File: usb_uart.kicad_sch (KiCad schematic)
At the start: 10 parts

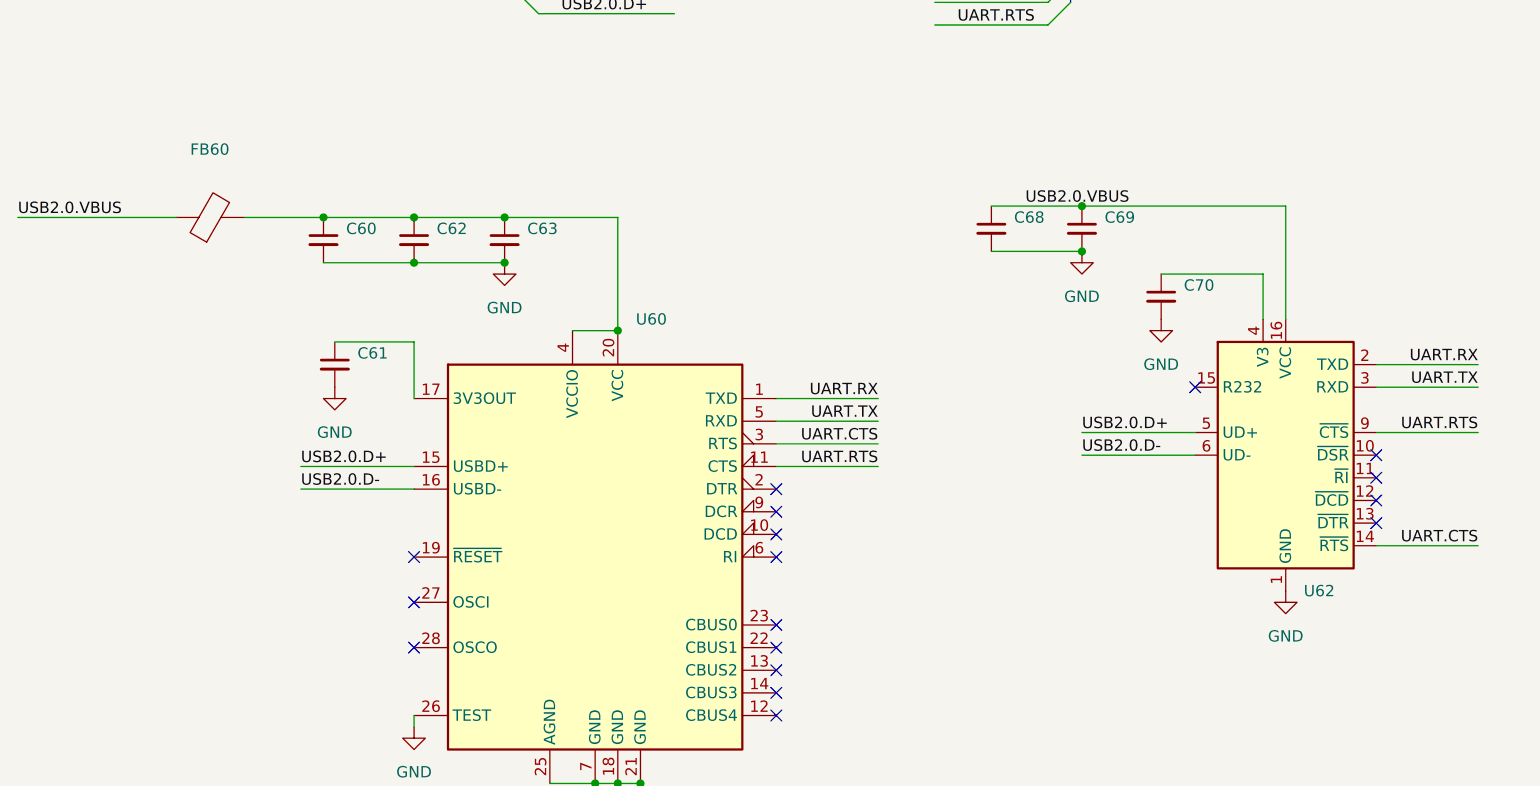
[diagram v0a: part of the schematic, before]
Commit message: Add heatsink, among other things
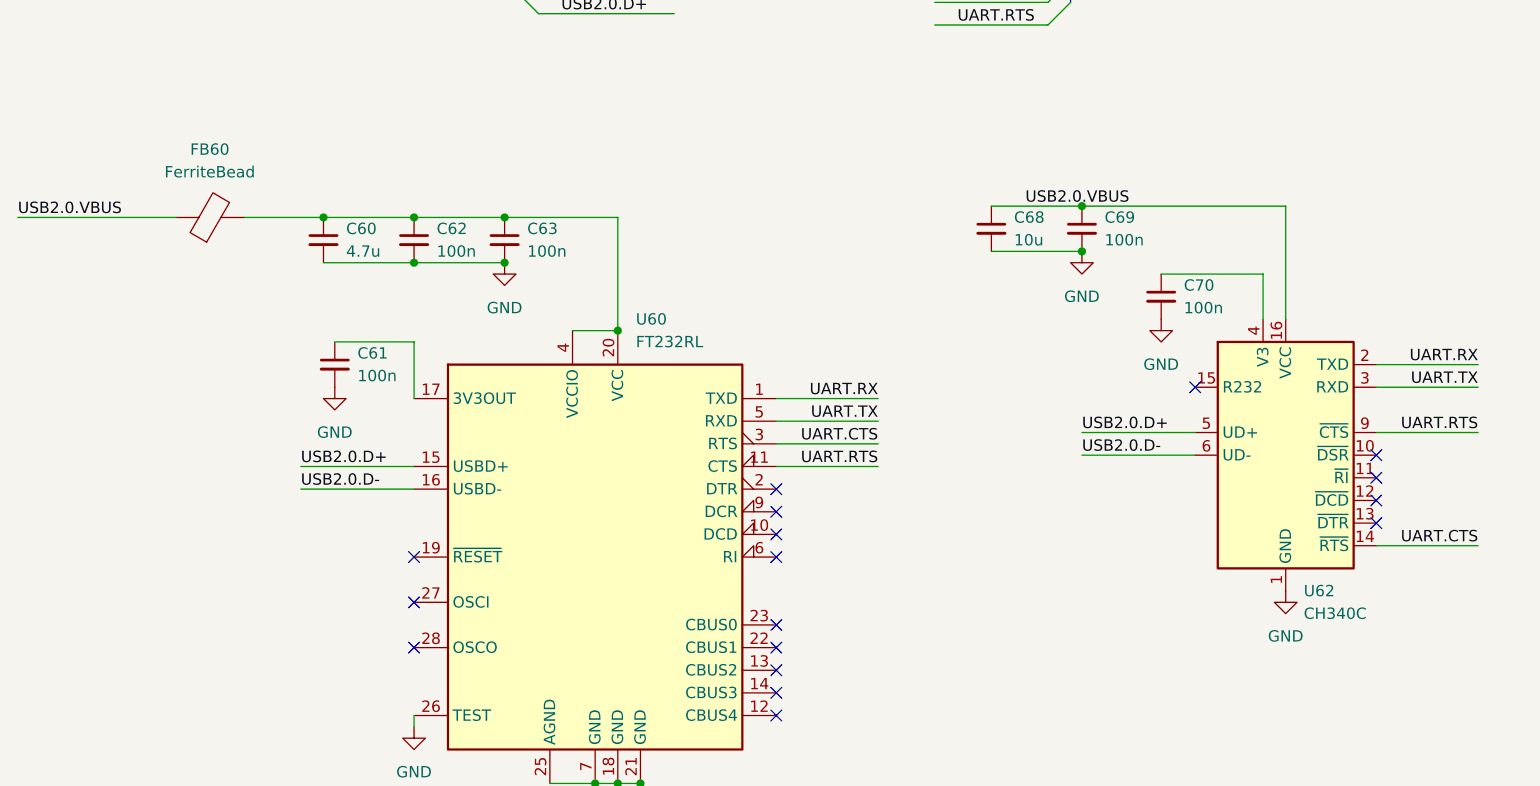
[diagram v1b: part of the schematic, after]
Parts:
- C60: value (none) -> 4.7u; footprint (none) -> Capacitor_SMD:C_0805_2012Metric
- C61, C62, C63, C69, C70: value (none) -> 100n; footprint (none) -> Capacitor_SMD:C_0402_1005Metric
- C68: value (none) -> 10u; footprint (none) -> Capacitor_SMD:C_0805_2012Metric
- FB60: value (none) -> FerriteBead; footprint (none) -> Inductor_SMD:L_0805_2012Metric
- U60: value (none) -> FT232RL; footprint (none) -> Package_SO:SSOP-28_5.3x10.2mm_P0.65mm
- U62: value (none) -> CH340C; footprint (none) -> Package_SO:SOIC-16_3.9x9.9mm_P1.27mm
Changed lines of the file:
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@@
       (effects (font (size 1.27 1.27)) (justify left))
     )
-    (property "Value" "" (id 1) (at 76.2 88.9062 0)
-      (effects (font (size 1.27 1.27)) (justify left))
-    )
-    (property "Footprint" "" (id 2) (at 73.66 87.63 0)
+    (property "Value" "100n" (id 1) (at 76.2 88.9062 0)
+      (effects (font (size 1.27 1.27)) (justify left))
+    )
+    (property "Footprint" "Capacitor_SMD:C_0402_1005Metric" (id 2) (at 73.66 87.63 0)
       (effects (font (size 1.27 1.27)) hide)
     )
@@
       (effects (font (size 1.27 1.27)) (justify left))
     )
-    (property "Value" "" (id 1) (at 107.4294 85.09 0)
-      (effects (font (size 1.27 1.27)) (justify left))
-    )
-    (property "Footprint" "" (id 2) (at 130.81 132.08 0)
+    (property "Value" "FT232RL" (id 1) (at 107.4294 85.09 0)
+      (effects (font (size 1.27 1.27)) (justify left))
+    )
+    (property "Footprint" "Package_SO:SSOP-28_5.3x10.2mm_P0.65mm" (id 2) (at 130.81 132.08 0)
       (effects (font (size 1.27 1.27)) hide)
     )
@@
       (effects (font (size 1.27 1.27)) (justify left))
     )
-    (property "Value" "" (id 1) (at 182.3594 115.57 0)
-      (effects (font (size 1.27 1.27)) (justify left))
-    )
-    (property "Footprint" "" (id 2) (at 181.61 111.76 0)
+    (property "Value" "CH340C" (id 1) (at 182.3594 115.57 0)
+      (effects (font (size 1.27 1.27)) (justify left))
+    )
+    (property "Footprint" "Package_SO:SOIC-16_3.9x9.9mm_P1.27mm" (id 2) (at 181.61 111.76 0)
       (effects (font (size 1.27 1.27)) (justify left) hide)
     )
@@
       (effects (font (size 1.27 1.27)) (justify left))
     )
-    (property "Value" "" (id 1) (at 85.09 74.9362 0)
-      (effects (font (size 1.27 1.27)) (justify left))
-    )
-    (property "Footprint" "" (id 2) (at 82.55 73.66 0)
+    (property "Value" "100n" (id 1) (at 85.09 74.9362 0)
+      (effects (font (size 1.27 1.27)) (justify left))
+    )
+    (property "Footprint" "Capacitor_SMD:C_0402_1005Metric" (id 2) (at 82.55 73.66 0)
       (effects (font (size 1.27 1.27)) hide)
     )
@@
       (effects (font (size 1.27 1.27)) (justify left))
     )
-    (property "Value" "" (id 1) (at 168.91 81.2862 0)
-      (effects (font (size 1.27 1.27)) (justify left))
-    )
-    (property "Footprint" "" (id 2) (at 166.37 80.01 0)
+    (property "Value" "100n" (id 1) (at 168.91 81.2862 0)
+      (effects (font (size 1.27 1.27)) (justify left))
+    )
+    (property "Footprint" "Capacitor_SMD:C_0402_1005Metric" (id 2) (at 166.37 80.01 0)
       (effects (font (size 1.27 1.27)) hide)
     )
@@
       (effects (font (size 1.27 1.27)) (justify left))
     )
-    (property "Value" "" (id 1) (at 149.86 73.6662 0)
-      (effects (font (size 1.27 1.27)) (justify left))
-    )
-    (property "Footprint" "" (id 2) (at 147.32 72.39 0)
+    (property "Value" "10u" (id 1) (at 149.86 73.6662 0)
+      (effects (font (size 1.27 1.27)) (justify left))
+    )
+    (property "Footprint" "Capacitor_SMD:C_0805_2012Metric" (id 2) (at 147.32 72.39 0)
       (effects (font (size 1.27 1.27)) hide)
     )
@@
       (effects (font (size 1.27 1.27)) (justify left))
     )
-    (property "Value" "" (id 1) (at 160.02 73.6662 0)
-      (effects (font (size 1.27 1.27)) (justify left))
-    )
-    (property "Footprint" "" (id 2) (at 157.48 72.39 0)
+    (property "Value" "100n" (id 1) (at 160.02 73.6662 0)
+      (effects (font (size 1.27 1.27)) (justify left))
+    )
+    (property "Footprint" "Capacitor_SMD:C_0402_1005Metric" (id 2) (at 157.48 72.39 0)
       (effects (font (size 1.27 1.27)) hide)
     )
@@
       (effects (font (size 1.27 1.27)) (justify left))
     )
-    (property "Value" "" (id 1) (at 95.25 74.9362 0)
-      (effects (font (size 1.27 1.27)) (justify left))
-    )
-    (property "Footprint" "" (id 2) (at 92.71 73.66 0)
+    (property "Value" "100n" (id 1) (at 95.25 74.9362 0)
+      (effects (font (size 1.27 1.27)) (justify left))
+    )
+    (property "Footprint" "Capacitor_SMD:C_0402_1005Metric" (id 2) (at 92.71 73.66 0)
       (effects (font (size 1.27 1.27)) hide)
     )
@@
       (effects (font (size 1.27 1.27)) (justify left))
     )
-    (property "Value" "" (id 1) (at 74.93 74.9362 0)
-      (effects (font (size 1.27 1.27)) (justify left))
-    )
-    (property "Footprint" "" (id 2) (at 72.39 73.66 0)
+    (property "Value" "4.7u" (id 1) (at 74.93 74.9362 0)
+      (effects (font (size 1.27 1.27)) (justify left))
+    )
+    (property "Footprint" "Capacitor_SMD:C_0805_2012Metric" (id 2) (at 72.39 73.66 0)
       (effects (font (size 1.27 1.27)) hide)
     )
@@
     (in_bom yes) (on_board yes) (fields_autoplaced)
     (property "Reference" "FB60" (id 0) (at 59.6392 63.5 90))
-    (property "Value" "" (id 1) (at 59.6392 66.04 90))
-    (property "Footprint" "" (id 2) (at 59.69 72.898 90)
-      (effects (font (size 1.27 1.27)) hide)
-    )
+    (property "Value" "FerriteBead" (id 1) (at 59.6392 66.04 90))
+    (property "Footprint" "Inductor_SMD:L_0805_2012Metric" (id 2) (at 59.69 72.898 90)
+      (effects (font (size 1.27 1.27)) hide)
+    )

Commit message: WIP PCB Routing
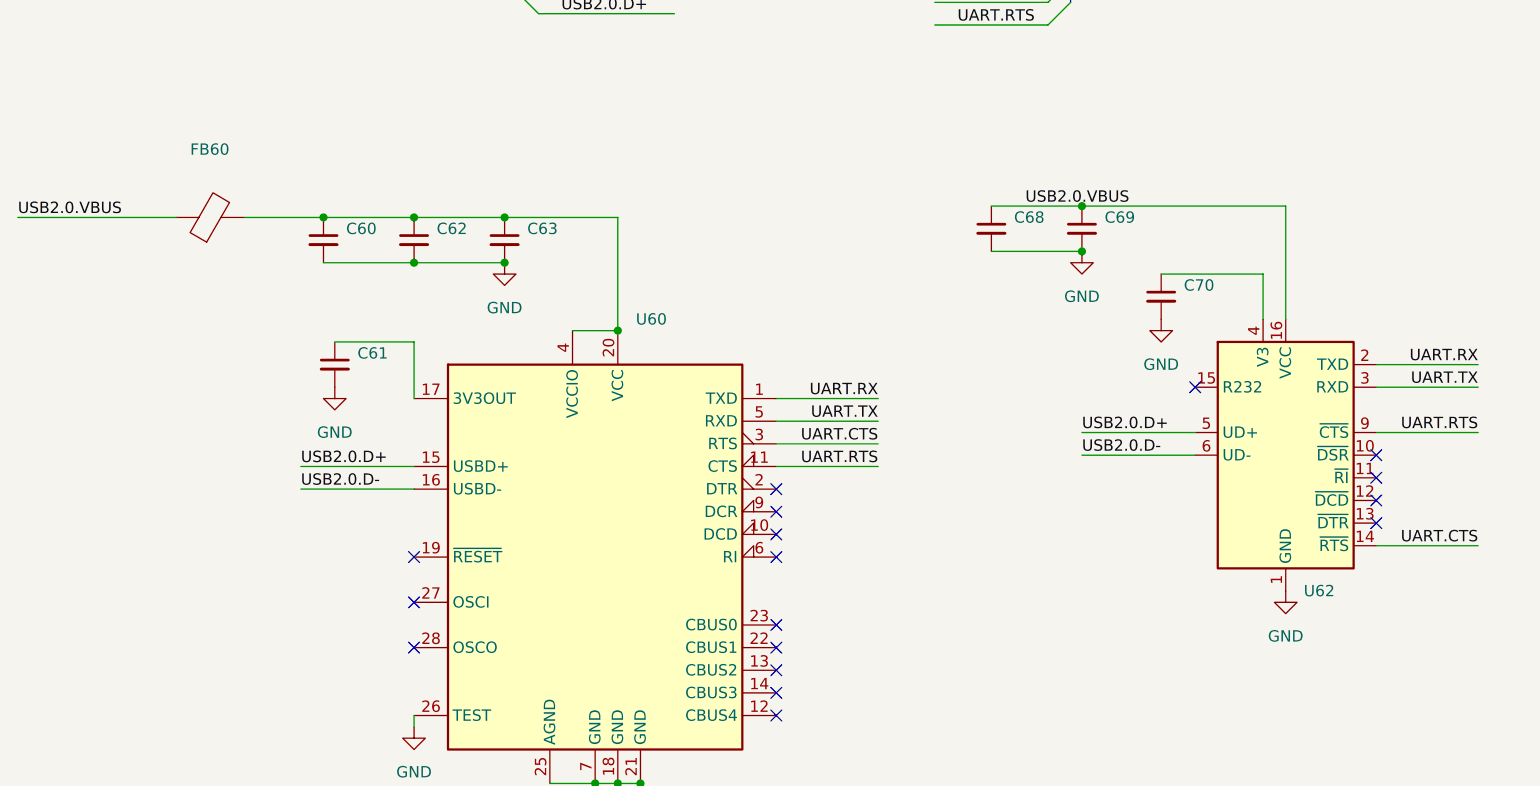
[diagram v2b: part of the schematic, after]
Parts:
- C60: value 4.7u -> (none); footprint Capacitor_SMD:C_0805_2012Metric -> (none)
- C61, C62, C63, C69, C70: value 100n -> (none); footprint Capacitor_SMD:C_0402_1005Metric -> (none)
- C68: value 10u -> (none); footprint Capacitor_SMD:C_0805_2012Metric -> (none)
- FB60: value FerriteBead -> (none); footprint Inductor_SMD:L_0805_2012Metric -> (none)
- U60: value FT232RL -> (none); footprint Package_SO:SSOP-28_5.3x10.2mm_P0.65mm -> (none)
- U62: value CH340C -> (none); footprint Package_SO:SOIC-16_3.9x9.9mm_P1.27mm -> (none)
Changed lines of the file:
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@@
       (effects (font (size 1.27 1.27)) (justify left))
     )
-    (property "Value" "100n" (id 1) (at 76.2 88.9062 0)
-      (effects (font (size 1.27 1.27)) (justify left))
-    )
-    (property "Footprint" "Capacitor_SMD:C_0402_1005Metric" (id 2) (at 73.66 87.63 0)
+    (property "Value" "" (id 1) (at 76.2 88.9062 0)
+      (effects (font (size 1.27 1.27)) (justify left))
+    )
+    (property "Footprint" "" (id 2) (at 73.66 87.63 0)
       (effects (font (size 1.27 1.27)) hide)
     )
@@
       (effects (font (size 1.27 1.27)) (justify left))
     )
-    (property "Value" "FT232RL" (id 1) (at 107.4294 85.09 0)
-      (effects (font (size 1.27 1.27)) (justify left))
-    )
-    (property "Footprint" "Package_SO:SSOP-28_5.3x10.2mm_P0.65mm" (id 2) (at 130.81 132.08 0)
+    (property "Value" "" (id 1) (at 107.4294 85.09 0)
+      (effects (font (size 1.27 1.27)) (justify left))
+    )
+    (property "Footprint" "" (id 2) (at 130.81 132.08 0)
       (effects (font (size 1.27 1.27)) hide)
     )
@@
       (effects (font (size 1.27 1.27)) (justify left))
     )
-    (property "Value" "CH340C" (id 1) (at 182.3594 115.57 0)
-      (effects (font (size 1.27 1.27)) (justify left))
-    )
-    (property "Footprint" "Package_SO:SOIC-16_3.9x9.9mm_P1.27mm" (id 2) (at 181.61 111.76 0)
+    (property "Value" "" (id 1) (at 182.3594 115.57 0)
+      (effects (font (size 1.27 1.27)) (justify left))
+    )
+    (property "Footprint" "" (id 2) (at 181.61 111.76 0)
       (effects (font (size 1.27 1.27)) (justify left) hide)
     )
@@
       (effects (font (size 1.27 1.27)) (justify left))
     )
-    (property "Value" "100n" (id 1) (at 85.09 74.9362 0)
-      (effects (font (size 1.27 1.27)) (justify left))
-    )
-    (property "Footprint" "Capacitor_SMD:C_0402_1005Metric" (id 2) (at 82.55 73.66 0)
+    (property "Value" "" (id 1) (at 85.09 74.9362 0)
+      (effects (font (size 1.27 1.27)) (justify left))
+    )
+    (property "Footprint" "" (id 2) (at 82.55 73.66 0)
       (effects (font (size 1.27 1.27)) hide)
     )
@@
       (effects (font (size 1.27 1.27)) (justify left))
     )
-    (property "Value" "100n" (id 1) (at 168.91 81.2862 0)
-      (effects (font (size 1.27 1.27)) (justify left))
-    )
-    (property "Footprint" "Capacitor_SMD:C_0402_1005Metric" (id 2) (at 166.37 80.01 0)
+    (property "Value" "" (id 1) (at 168.91 81.2862 0)
+      (effects (font (size 1.27 1.27)) (justify left))
+    )
+    (property "Footprint" "" (id 2) (at 166.37 80.01 0)
       (effects (font (size 1.27 1.27)) hide)
     )
@@
       (effects (font (size 1.27 1.27)) (justify left))
     )
-    (property "Value" "10u" (id 1) (at 149.86 73.6662 0)
-      (effects (font (size 1.27 1.27)) (justify left))
-    )
-    (property "Footprint" "Capacitor_SMD:C_0805_2012Metric" (id 2) (at 147.32 72.39 0)
+    (property "Value" "" (id 1) (at 149.86 73.6662 0)
+      (effects (font (size 1.27 1.27)) (justify left))
+    )
+    (property "Footprint" "" (id 2) (at 147.32 72.39 0)
       (effects (font (size 1.27 1.27)) hide)
     )
@@
       (effects (font (size 1.27 1.27)) (justify left))
     )
-    (property "Value" "100n" (id 1) (at 160.02 73.6662 0)
-      (effects (font (size 1.27 1.27)) (justify left))
-    )
-    (property "Footprint" "Capacitor_SMD:C_0402_1005Metric" (id 2) (at 157.48 72.39 0)
+    (property "Value" "" (id 1) (at 160.02 73.6662 0)
+      (effects (font (size 1.27 1.27)) (justify left))
+    )
+    (property "Footprint" "" (id 2) (at 157.48 72.39 0)
       (effects (font (size 1.27 1.27)) hide)
     )
@@
       (effects (font (size 1.27 1.27)) (justify left))
     )
-    (property "Value" "100n" (id 1) (at 95.25 74.9362 0)
-      (effects (font (size 1.27 1.27)) (justify left))
-    )
-    (property "Footprint" "Capacitor_SMD:C_0402_1005Metric" (id 2) (at 92.71 73.66 0)
+    (property "Value" "" (id 1) (at 95.25 74.9362 0)
+      (effects (font (size 1.27 1.27)) (justify left))
+    )
+    (property "Footprint" "" (id 2) (at 92.71 73.66 0)
       (effects (font (size 1.27 1.27)) hide)
     )
@@
       (effects (font (size 1.27 1.27)) (justify left))
     )
-    (property "Value" "4.7u" (id 1) (at 74.93 74.9362 0)
-      (effects (font (size 1.27 1.27)) (justify left))
-    )
-    (property "Footprint" "Capacitor_SMD:C_0805_2012Metric" (id 2) (at 72.39 73.66 0)
+    (property "Value" "" (id 1) (at 74.93 74.9362 0)
+      (effects (font (size 1.27 1.27)) (justify left))
+    )
+    (property "Footprint" "" (id 2) (at 72.39 73.66 0)
       (effects (font (size 1.27 1.27)) hide)
     )
@@
     (in_bom yes) (on_board yes) (fields_autoplaced)
     (property "Reference" "FB60" (id 0) (at 59.6392 63.5 90))
-    (property "Value" "FerriteBead" (id 1) (at 59.6392 66.04 90))
-    (property "Footprint" "Inductor_SMD:L_0805_2012Metric" (id 2) (at 59.69 72.898 90)
-      (effects (font (size 1.27 1.27)) hide)
-    )
+    (property "Value" "" (id 1) (at 59.6392 66.04 90))
+    (property "Footprint" "" (id 2) (at 59.69 72.898 90)
+      (effects (font (size 1.27 1.27)) hide)
+    )
